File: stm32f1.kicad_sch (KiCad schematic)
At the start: 19 parts, among them SW1 SW_Push, SW2 SW_Push, U1 STM32F103C8Tx

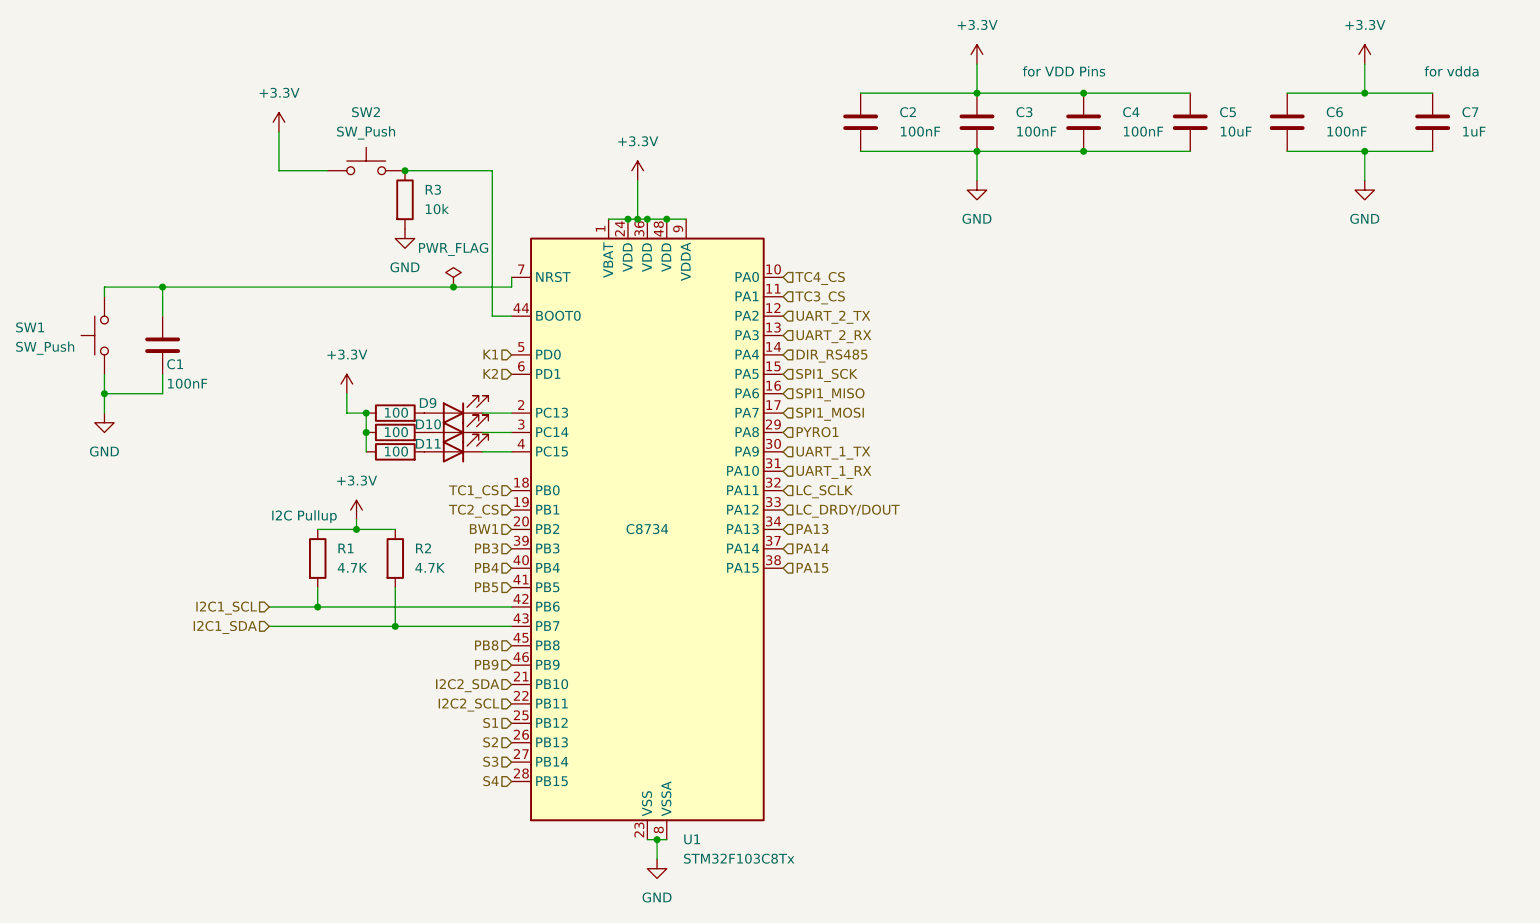
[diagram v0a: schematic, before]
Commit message: Initial pass at finding Mouser part numbers
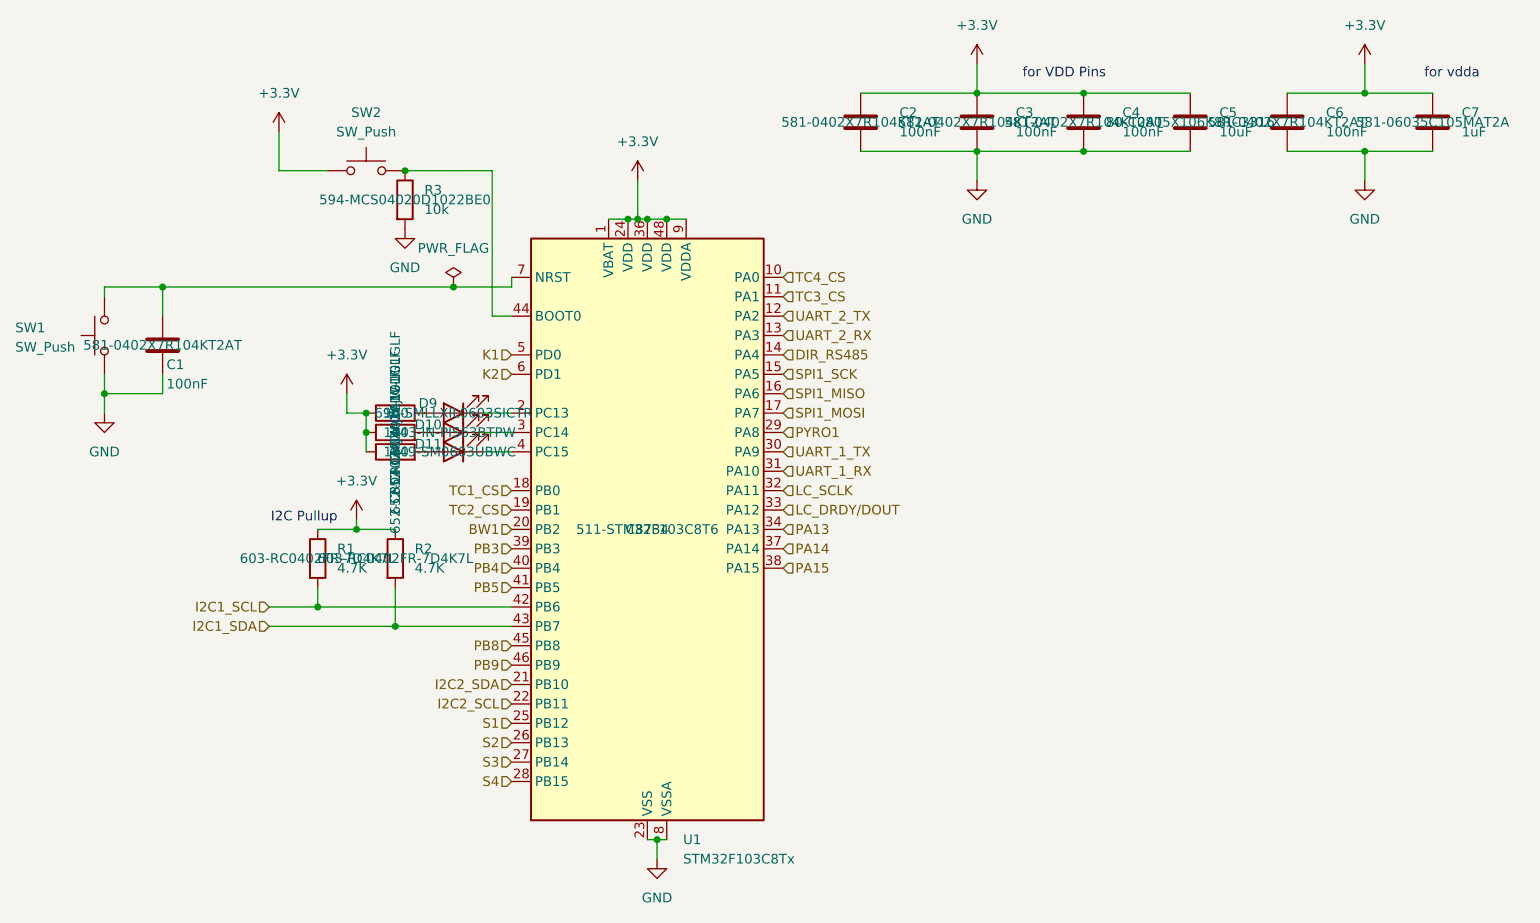
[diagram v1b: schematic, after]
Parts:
- C1, C2, C3, C4, C6: Mouser Part Number  (none) -> 581-0402X7R104KT2AT
- C5: Mouser Part Number  (none) -> 80-C0805X106K8RC3316
- C7: Mouser Part Number  (none) -> 581-06035C105MAT2A
- D10: Mouser Part Number  (none) -> 743-IN-PIS63BTPW
- D11: Mouser Part Number  (none) -> 749-SM0603UBWC
- D9: Mouser Part Number  (none) -> 696-SMLLXIL0603SICTR
- R1, R2: Mouser Part Number  (none) -> 603-RC0402FR-7D4K7L
- R28, R29, R30: Mouser Part Number  (none) -> 652-CR0402AJW-101GLF
- R3: Mouser Part Number  (none) -> 594-MCS04020D1022BE0
- U1: Mouser Part Number  (none) -> 511-STM32F103C8T6
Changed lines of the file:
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@@
+			)
+		)
+		(property "Mouser Part Number " "652-CR0402AJW-101GLF "
+			(at 107.95 93.98 0)
+			(effects
+				(font
+					(size 1.27 1.27)
+				)
 			)
 		)
@@
 			)
 		)
+		(property "Mouser Part Number " "581-0402X7R104KT2AT "
+			(at 184.15 50.8 0)
+			(effects
+				(font
+					(size 1.27 1.27)
+				)
+			)
+		)
 		(pin "1"
 		)
@@
 			)
 		)
+		(property "Mouser Part Number " "749-SM0603UBWC "
+			(at 115.57 93.98 0)
+			(effects
+				(font
+					(size 1.27 1.27)
+				)
+			)
+		)
 		(pin "1"
 		)
@@
 		)
 		(property "JLC#" ""
+			(at 107.95 91.44 0)
+			(effects
+				(font
+					(size 1.27 1.27)
+				)
+			)
+		)
+		(property "Mouser Part Number " "652-CR0402AJW-101GLF "
 			(at 107.95 91.44 0)
 			(effects
@@
 			)
 		)
+		(property "Mouser Part Number " "603-RC0402FR-7D4K7L "
+			(at 97.79 107.95 0)
+			(effects
+				(font
+					(size 1.27 1.27)
+				)
+			)
+		)
 		(pin "1"
 		)
@@
 		)
 		(property "JLC#" ""
+			(at 77.47 80.01 0)
+			(effects
+				(font
+					(size 1.27 1.27)
+				)
+			)
+		)
+		(property "Mouser Part Number " "581-0402X7R104KT2AT "
 			(at 77.47 80.01 0)
 			(effects
@@
 			)
 		)
+		(property "Mouser Part Number " "696-SMLLXIL0603SICTR "
+			(at 115.57 88.9 0)
+			(effects
+				(font
+					(size 1.27 1.27)
+				)
+			)
+		)
 		(pin "1"
 		)
@@
 				)
 				(hide yes)
+			)
+		)
+		(property "Mouser Part Number " ""
+			(at 104.14 57.15 0)
+			(effects
+				(font
+					(size 1.27 1.27)
+				)
 			)
 		)
@@
 			)
 		)
+		(property "Mouser Part Number " "603-RC0402FR-7D4K7L "
+			(at 107.95 107.95 0)
+			(effects
+				(font
+					(size 1.27 1.27)
+				)
+			)
+		)
 		(pin "1"
 		)
@@
 			)
 		)
+		(property "Mouser Part Number " "743-IN-PIS63BTPW "
+			(at 115.57 91.44 0)
+			(effects
+				(font
+					(size 1.27 1.27)
+				)
+			)
+		)
 		(pin "1"
 		)
@@
 			)
 		)
+		(property "Mouser Part Number " "80-C0805X106K8RC3316 "
+			(at 212.09 50.8 0)
+			(effects
+				(font
+					(size 1.27 1.27)
+				)
+			)
+		)
 		(pin "1"
 		)
@@
 			)
 		)
+		(property "Mouser Part Number " "511-STM32F103C8T6 "
+			(at 140.97 104.14 0)
+			(effects
+				(font
+					(size 1.27 1.27)
+				)
+			)
+		)
 		(pin "7"
 		)
@@
 			)
 		)
+		(property "Mouser Part Number " "581-0402X7R104KT2AT "
+			(at 224.79 50.8 0)
+			(effects
+				(font
+					(size 1.27 1.27)
+				)
+			)
+		)
 		(pin "1"
 		)
@@
 			)
 		)
+		(property "Mouser Part Number " ""
+			(at 69.85 78.74 0)
+			(effects
+				(font
+					(size 1.27 1.27)
+				)
+			)
+		)
 		(pin "1"
 		)
@@
 		)
 		(property "JLC#" ""
+			(at 198.12 50.8 0)
+			(effects
+				(font
+					(size 1.27 1.27)
+				)
+			)
+		)
+		(property "Mouser Part Number " "581-0402X7R104KT2AT "
 			(at 198.12 50.8 0)
 			(effects
@@
 			)
 		)
+		(property "Mouser Part Number " "594-MCS04020D1022BE0 "
+			(at 109.22 60.96 0)
+			(effects
+				(font
+					(size 1.27 1.27)
+				)
+			)
+		)
 		(pin "2"
 		)
@@
 		)
 		(property "JLC#" ""
+			(at 107.95 88.9 0)
+			(effects
+				(font
+					(size 1.27 1.27)
+				)
+			)
+		)
+		(property "Mouser Part Number " "652-CR0402AJW-101GLF "
 			(at 107.95 88.9 0)
 			(effects
@@
 			)
 		)
+		(property "Mouser Part Number " "581-0402X7R104KT2AT "
+			(at 168.91 50.8 0)
+			(effects
+				(font
+					(size 1.27 1.27)
+				)
+			)
+		)
 		(pin "1"
 		)
@@
 			(at 243.84 50.8 0)
 			(effects
+				(font
+					(size 1.27 1.27)
+				)
+			)
+		)
+		(property "Mouser Part Number " "581-06035C105MAT2A "
+			(at 243.84 50.8 0)
+			(effects
